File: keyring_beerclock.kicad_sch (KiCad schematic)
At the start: 39 parts, among them J1 +BAT, J2 -BAT, J3 VCC, J4 UDPI, J5 GND, J6 +PIEZO, J7 -PIEZO, J8 USB_C_Receptacle_USB2.0, SW1 PWR_SEL, SW2 BTN_LEFT, SW3 BTN_RIGHT, SW4 BTN_MID, U1 SSD1306-14pin, U2 MCP73812T-420I-OT, U3 TC1014-3.3VCT713, U4 ATtiny1616-MNR

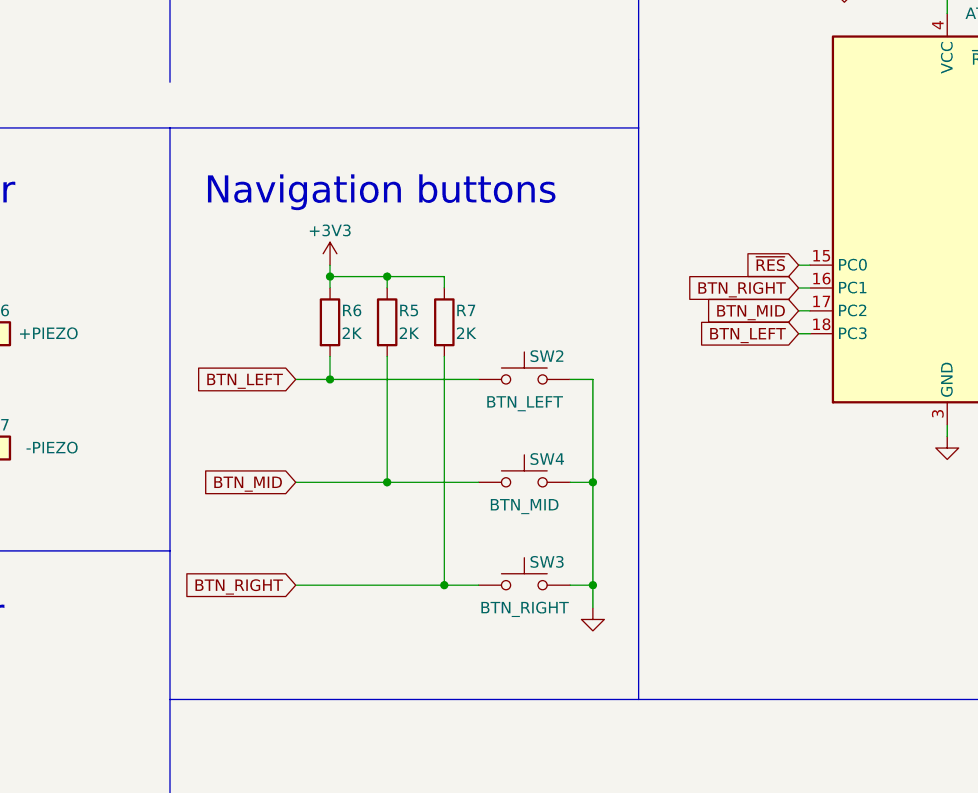
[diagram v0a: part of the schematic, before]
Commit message: Finished layout, ready to order
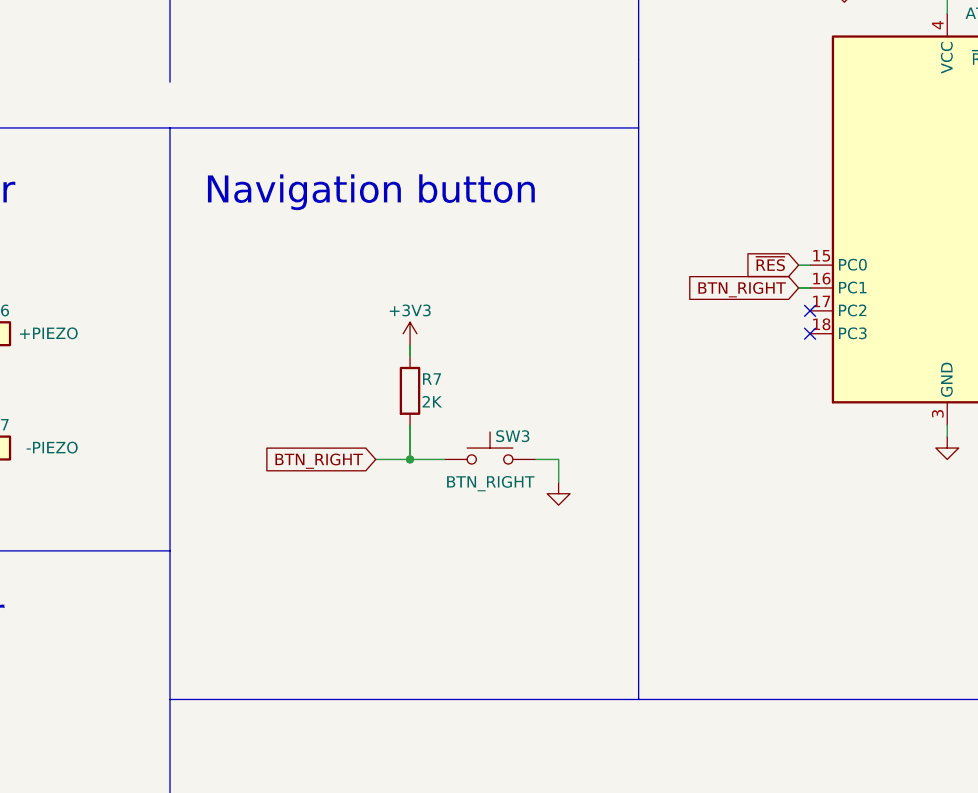
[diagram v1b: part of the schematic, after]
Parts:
- removed R5, R6: 2K, Resistor_SMD:R_0402_1005Metric_Pad0.72x0.64mm_HandSolder, symbol Device:R
- removed SW2: BTN_LEFT, Button_Switch_SMD:SW_SPST_B3U-1000P, symbol Switch:SW_Push
- removed SW4: BTN_MID, Button_Switch_SMD:SW_SPST_B3U-1000P, symbol Switch:SW_Push
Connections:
- net BTN_LEFT: no longer names the net of U4.18 (PC3)
- net BTN_MID: no longer names the net of U4.17 (PC2)
- no-connect marks 18 -> 20
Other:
- note added: "Navigation button"
- note removed: "Navigation buttons"
- moved on the sheet: R7, SW3
